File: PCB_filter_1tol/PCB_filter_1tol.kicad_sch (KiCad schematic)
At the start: 26 parts, among them J1 Conn_01x02_Pin, J2 Conn_01x02_Pin, U1 AD620, U2 LM324

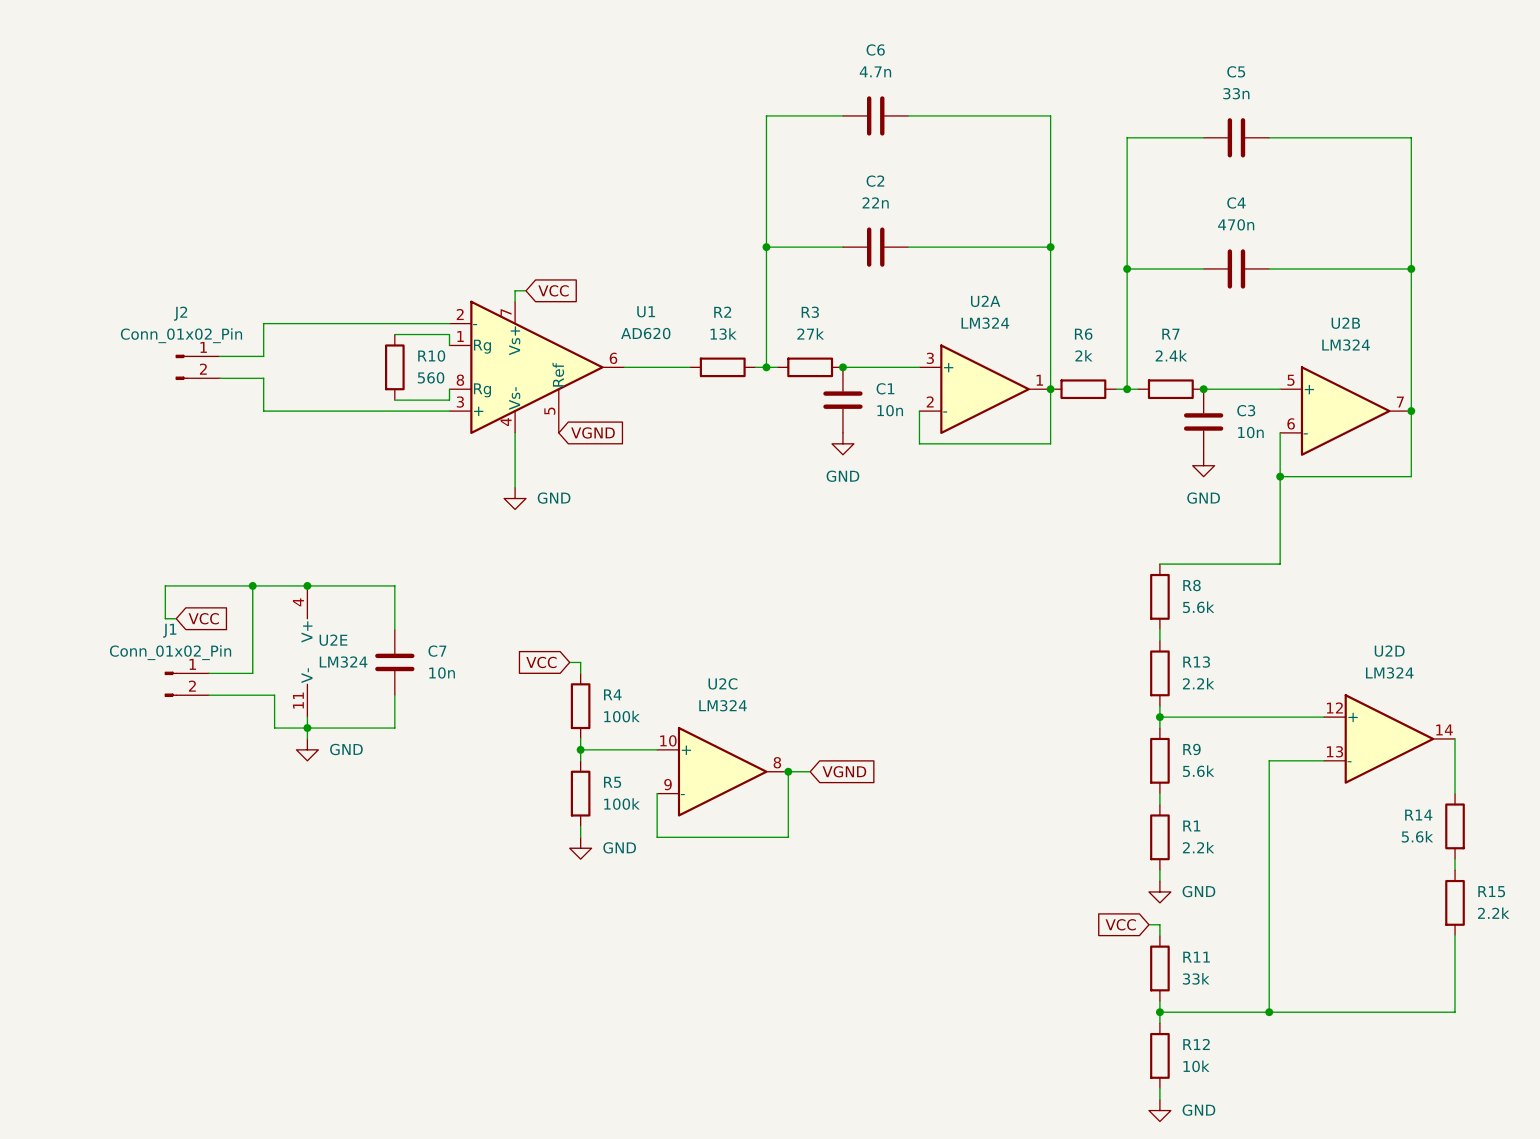
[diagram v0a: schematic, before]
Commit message: last
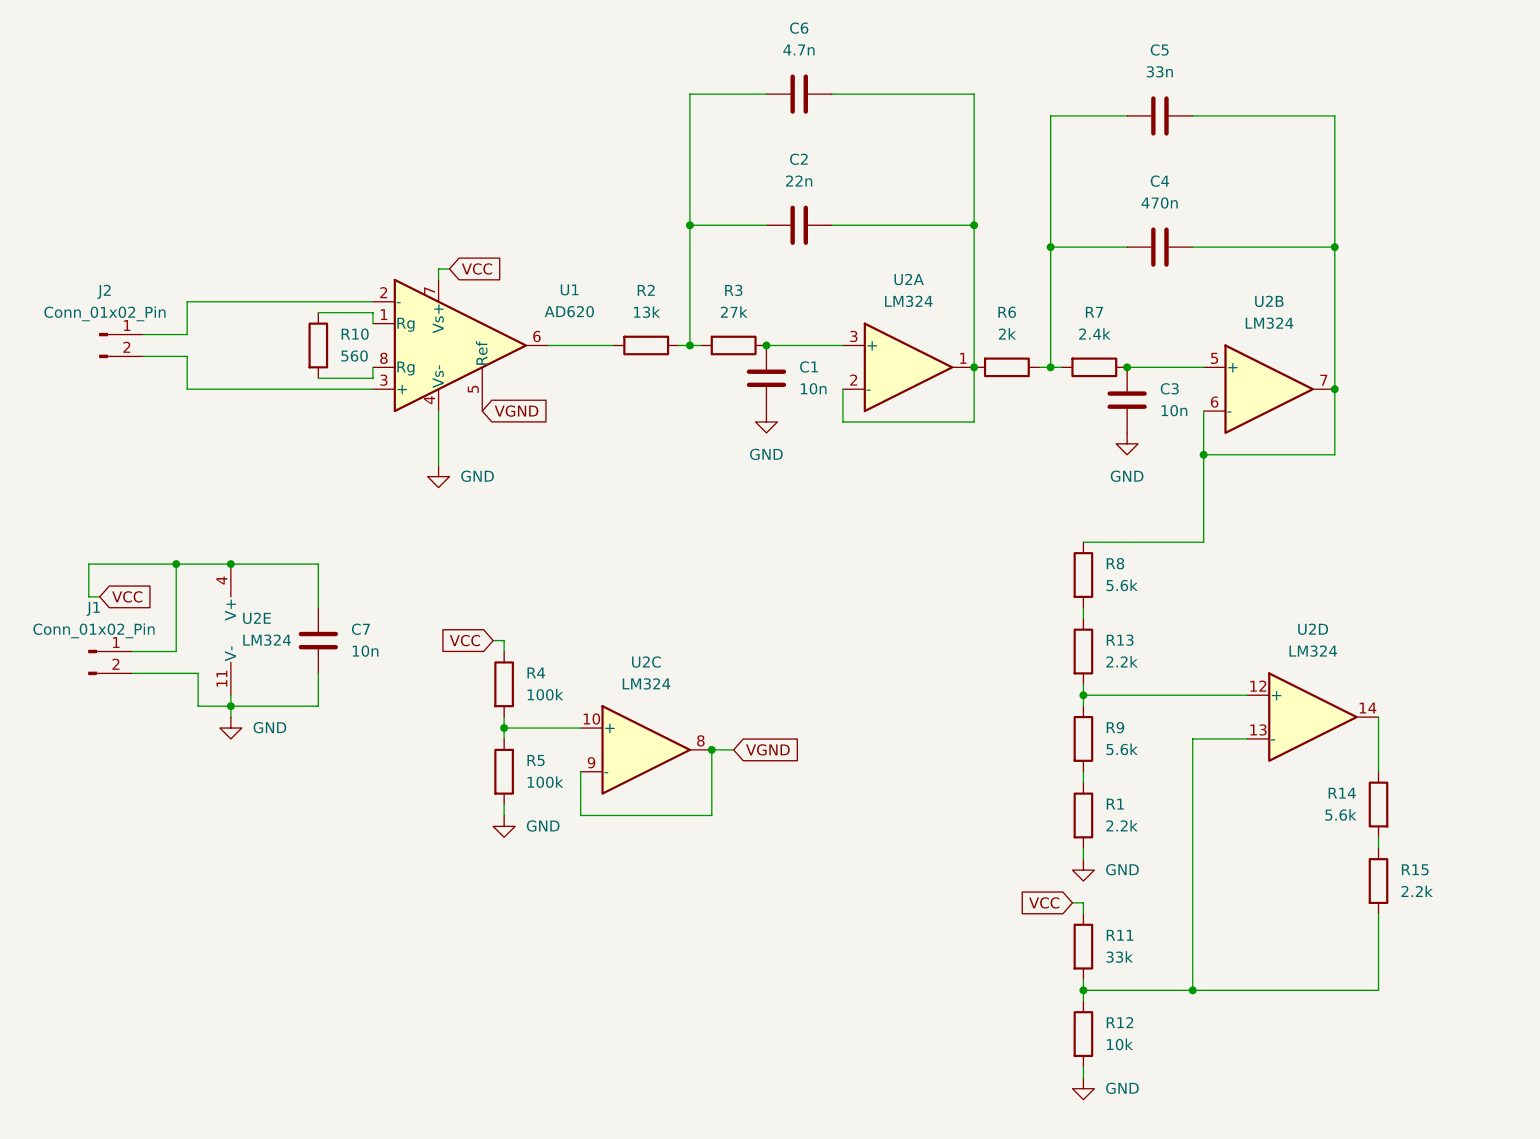
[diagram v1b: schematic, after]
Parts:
- C1, C2, C3, C4, C5, C6, C7: footprint Capacitor_SMD:C_0805_2012Metric_Pad1.18x1.45mm_HandSolder -> Capacitor_THT:C_Disc_D5.0mm_W2.5mm_P2.50mm
- R1, R10, R11, R12, R13, R14, R15, R2, R3, R4, R5, R6, R7, R8, R9: footprint Resistor_SMD:R_0805_2012Metric_Pad1.20x1.40mm_HandSolder -> Resistor_THT:R_Axial_DIN0207_L6.3mm_D2.5mm_P7.62mm_Horizontal
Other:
- moved on the sheet: C1, C2, C3, C4, C5, C6, C7, J1, J2, R1, R10, R11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
